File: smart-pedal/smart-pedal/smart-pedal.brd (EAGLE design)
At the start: 20.3 x 25.4 mm, 18 parts, among them Q1 MMBT5088

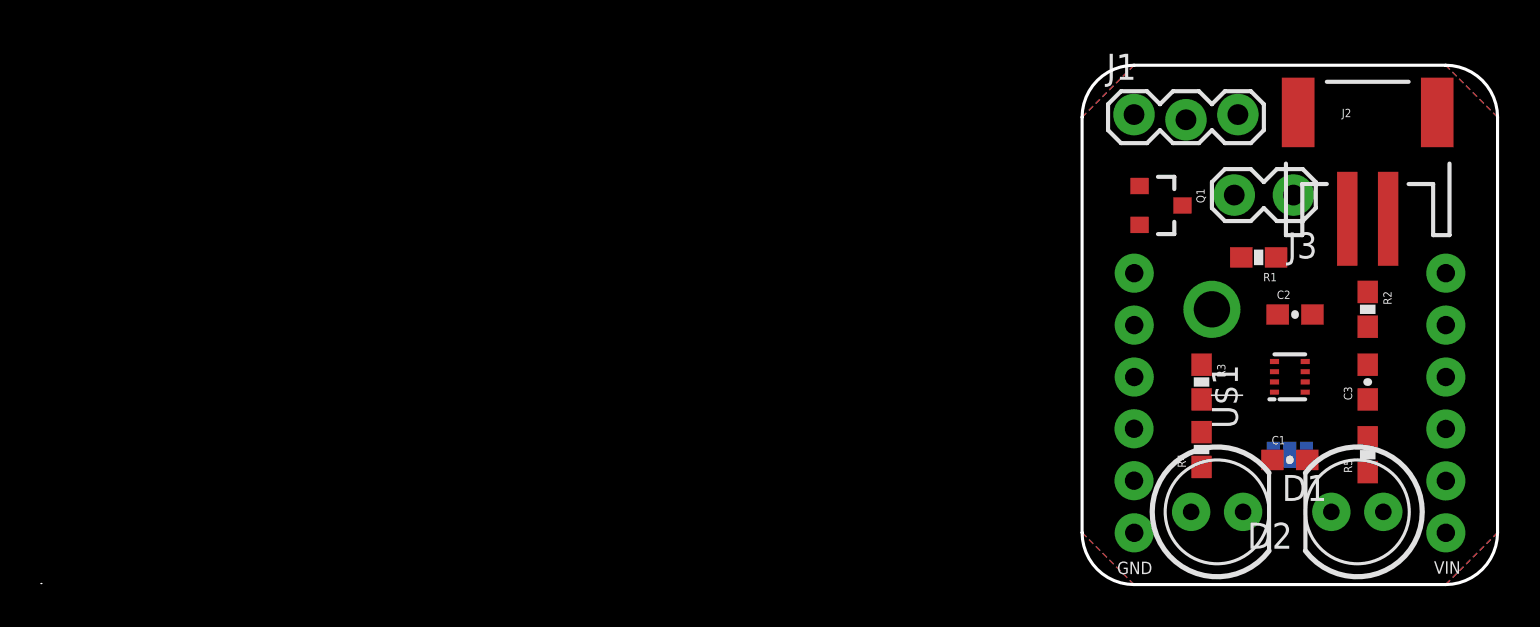
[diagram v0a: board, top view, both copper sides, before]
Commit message: cleanup
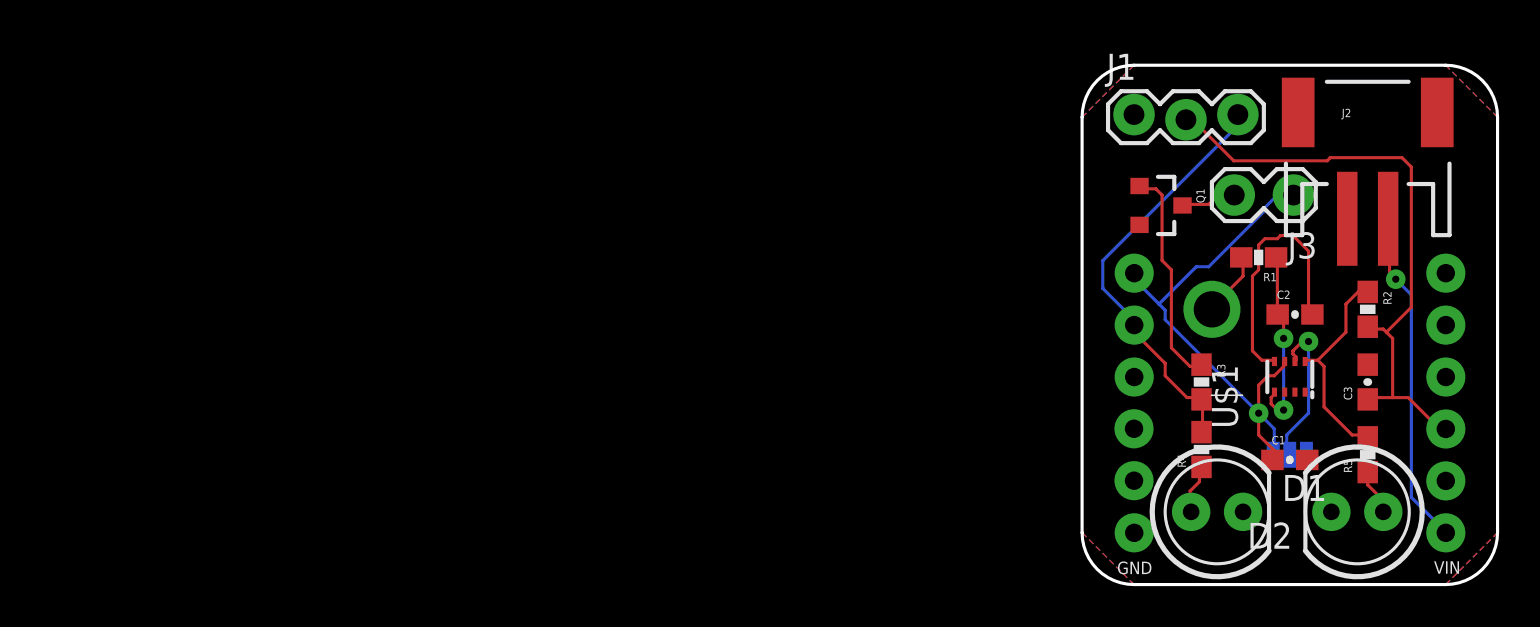
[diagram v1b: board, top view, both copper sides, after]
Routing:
- net OUT_FILTERED: track 0.00 -> 29.6 mm
- net VDD: track 0.00 -> 26.5 mm, vias 0 -> 1
- net MOTOR_OUT: track 0.00 -> 20.9 mm
- net V_BATT: track 0.00 -> 16.5 mm, vias 0 -> 1
- net SNS: track 0.00 -> 12.7 mm
- net N$2: track 0.00 -> 10.9 mm
- net OUT: track 0.00 -> 10.5 mm
- net SNSK: track 0.00 -> 9.04 mm, vias 0 -> 2
- net SYNC: track 0.00 -> 7.60 mm, vias 0 -> 1
- net CAP: track 0.00 -> 3.26 mm
- net N$1: track 0.00 -> 2.74 mm
- net N$4: track 0.00 -> 2.44 mm
- net N$5: track 0.00 -> 2.26 mm
